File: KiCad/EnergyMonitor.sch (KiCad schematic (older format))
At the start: 48 parts, among them J1 Conn_01x02, J10 4P4C, J2 AudioJack3_Ground_SwitchTR, J3 AudioJack3_Ground_SwitchTR, J4 AudioJack3_Ground_SwitchTR, J5 Conn_01x02, J6 Conn_01x02, J7 Conn_01x02, J8 Barrel_Jack_Switch, J9 Conn_01x04, U2 ESP32_D1_MINI, U3 HT7333

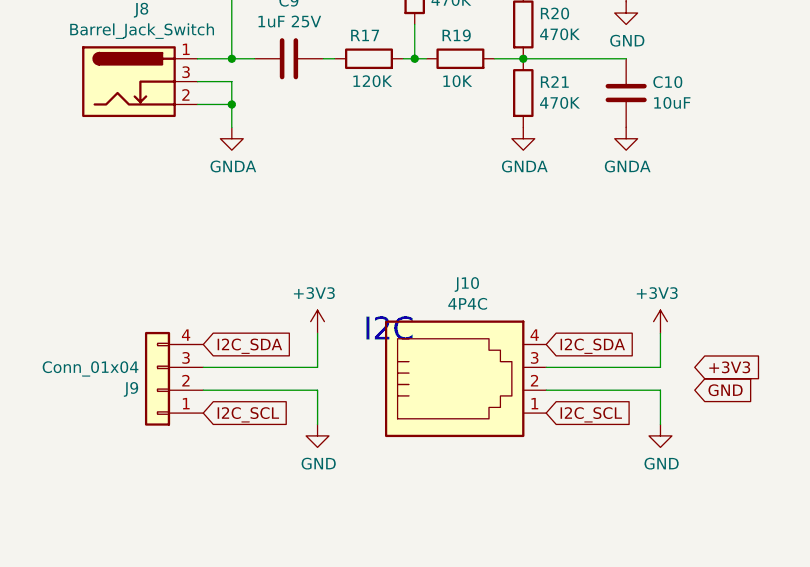
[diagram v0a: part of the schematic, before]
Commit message: pcb footprints
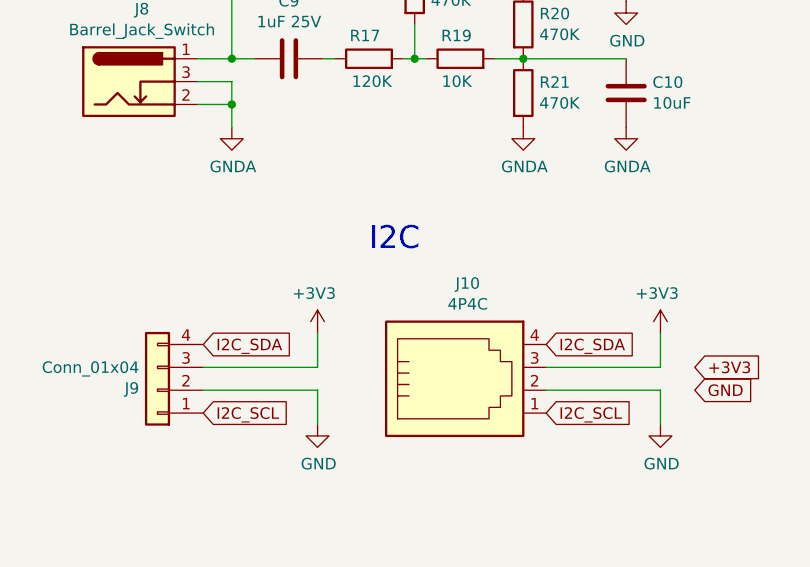
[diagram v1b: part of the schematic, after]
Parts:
- J2, J3, J4: footprint (none) -> MyFootprints:3.5mm_5_Pin_Socket_PCB_Mount
- J8: footprint (none) -> MyFootprints:DC_Barrel_Jack_Socket
- U2: footprint (none) -> MyFootprints:ESP32_D1_MINI
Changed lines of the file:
@@
 Sheet 1 1
 Title "ESP32 Energy Monitor"
-Date "2021-09-06"
+Date "2021-09-07"
 Rev "v1.0"
 Comp ""
@@
 F 0 "J8" H 7932 2517 50  0000 C CNN
 F 1 "Barrel_Jack_Switch" H 7932 2426 50  0000 C CNN
-F 2 "" H 7925 2160 50  0001 C CNN
+F 2 "MyFootprints:DC_Barrel_Jack_Socket" H 7925 2160 50  0001 C CNN
 F 3 "~" H 7925 2160 50  0001 C CNN
 	1    7875 2200
@@
 F 0 "U2" H 2050 3800 50  0000 C CNN
 F 1 "ESP32_D1_MINI" H 2050 4000 100 0000 C CNN
-F 2 "" H 2050 3125 50  0001 C CNN
+F 2 "MyFootprints:ESP32_D1_MINI" H 2050 3125 50  0001 C CNN
 F 3 "" H 2050 3125 50  0001 C CNN
 	1    2050 2675
@@
 F 0 "J2" H 4232 2325 50  0000 C CNN
 F 1 "AudioJack3_Ground_SwitchTR" H 4232 2234 50  0000 C CNN
-F 2 "" H 4250 2000 50  0001 C CNN
+F 2 "MyFootprints:3.5mm_5_Pin_Socket_PCB_Mount" H 4250 2000 50  0001 C CNN
 F 3 "~" H 4250 2000 50  0001 C CNN
 	1    4250 2000
@@
 F 0 "J3" H 4232 3775 50  0000 C CNN
 F 1 "AudioJack3_Ground_SwitchTR" H 4232 3684 50  0000 C CNN
-F 2 "" H 4250 3450 50  0001 C CNN
+F 2 "MyFootprints:3.5mm_5_Pin_Socket_PCB_Mount" H 4250 3450 50  0001 C CNN
 F 3 "~" H 4250 3450 50  0001 C CNN
 	1    4250 3450
@@
 F 0 "J4" H 4232 5225 50  0000 C CNN
 F 1 "AudioJack3_Ground_SwitchTR" H 4232 5134 50  0000 C CNN
-F 2 "" H 4250 4900 50  0001 C CNN
+F 2 "MyFootprints:3.5mm_5_Pin_Socket_PCB_Mount" H 4250 4900 50  0001 C CNN
 F 3 "~" H 4250 4900 50  0001 C CNN
 	1    4250 4900
@@
 	5650 4450 5650 4500
 Connection ~ 6500 4450
-Text Notes 8900 3350 0    100  ~ 0
+Text Notes 8925 2950 0    100  ~ 0
 I2C
 $EndSCHEMATC
